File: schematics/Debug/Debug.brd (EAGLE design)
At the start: 100 x 80 mm, 12 parts

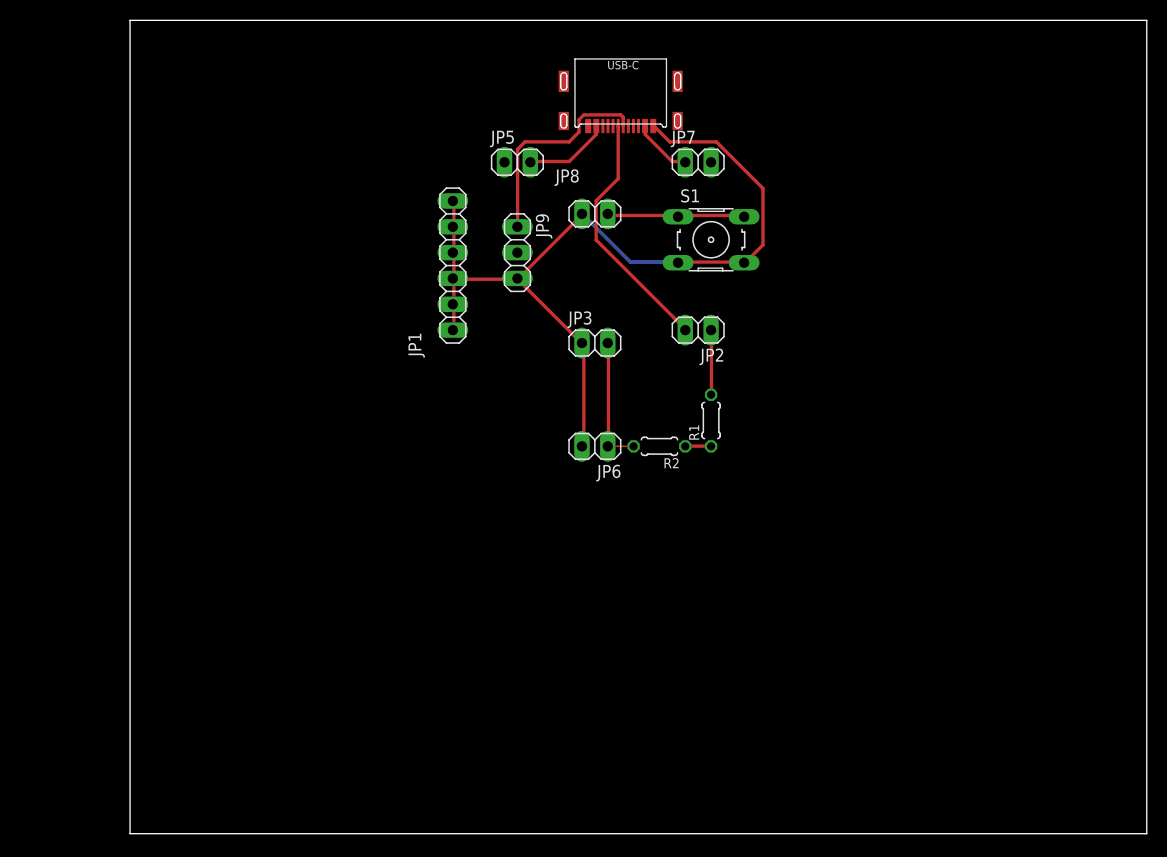
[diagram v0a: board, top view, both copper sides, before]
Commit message: Debug plata
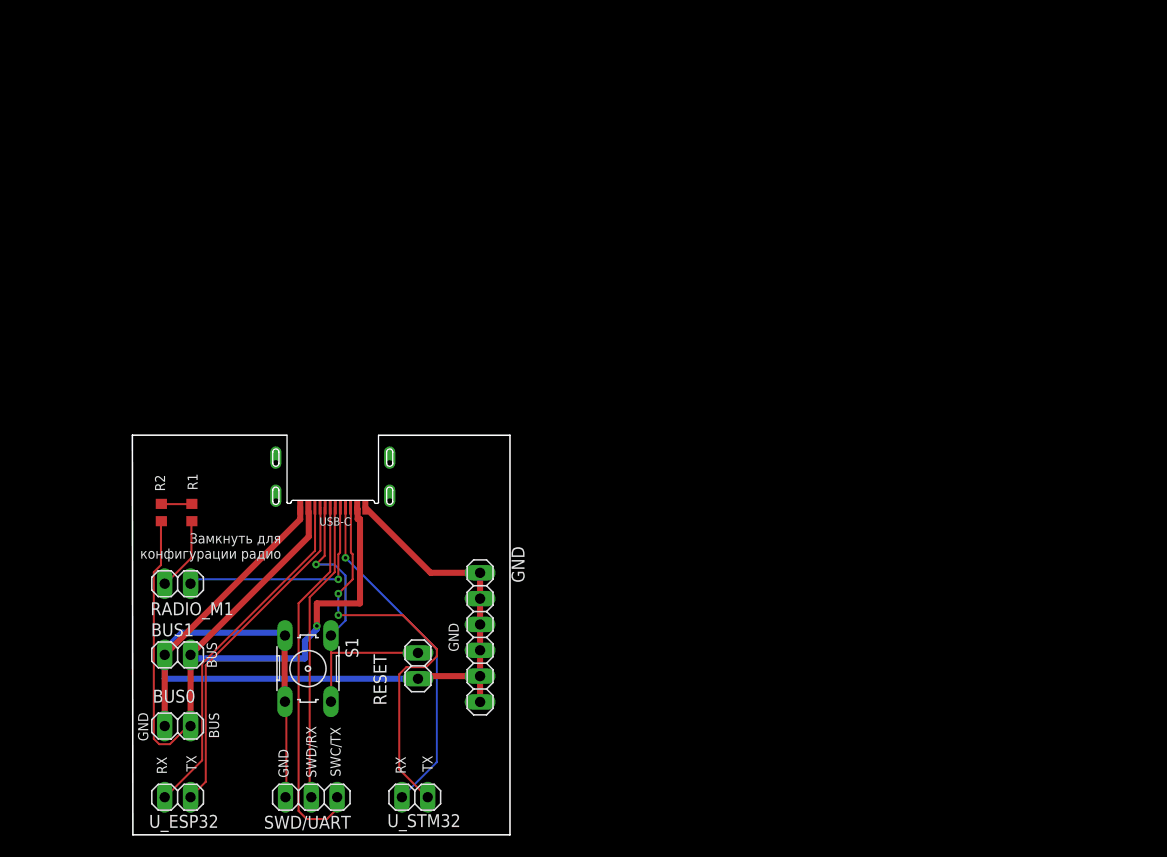
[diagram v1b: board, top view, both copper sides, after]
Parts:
- removed JP1: (no value), pinhead:1X06
- removed JP2, JP3, JP5, JP6, JP7, JP8: (no value), pinhead:1X02
- removed JP9: (no value), pinhead:1X03
- added BUS0, BUS1, RADIO_M1, RESET, U_ESP32, U_STM32: (no value), pinhead:1X02
- added GND: (no value), pinhead:1X06
- added SWD/UART: (no value), pinhead:1X03
- R1, R2: device resistor:0204/5 -> rcl:R0603
- moved S1 57.9 mm to (17.5, 16.2), turned to 270 degrees
- moved R1 51.9 mm to (6.08, 31.6), turned to 270 degrees
- moved R2 49.4 mm to (3.08, 31.6), turned to 270 degrees
- moved U$1 46.6 mm to (19.9, 39.2)
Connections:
- removed net N$1: JP5.2, U$1.TX1
- removed net N$10: JP1.1, JP1.2, JP1.3, JP1.4, JP1.5, JP1.6, JP3.1, JP6.2, JP8.1, JP9.3, S1.3, S1.4, U$1.GND0, U$1.GND1
- removed net N$11: JP9.2, U$1.SWDIO
- removed net N$12: JP9.1, U$1.SWDCLK
- removed net N$2: JP5.1, U$1.RX1
- removed net N$3: JP7.1, U$1.RX0
- removed net N$4: JP8.2, S1.1, S1.2, U$1.P$6
- removed net N$5: JP7.2, U$1.TX0
- removed net N$6: JP3.2, JP6.1, R2.2, U$1.VBUS0, U$1.VBUS1
- removed net N$9: JP2.2, U$1.M1
- new net BUS: BUS0.1, BUS1.2, R2.2, U$1.BUS0, U$1.BUS1
- new net GND: BUS0.2, BUS1.1, GND.1, GND.2, GND.3, GND.4, GND.5, GND.6, RESET.1, S1.3, S1.4, SWD/UART.3, U$1.GND0, U$1.GND1
- new net M1: RADIO_M1.2, U$1.M1
- new net RESET: RESET.2, S1.1, S1.2, U$1.RESET
- new net RX+: U$1.RX1, U_ESP32.1
- new net RX-: U$1.RX0, U_STM32.1
- new net SWC: SWD/UART.1, U$1.SWC
- new net SWD: SWD/UART.2, U$1.SWD
- new net TX+: U$1.TX1, U_ESP32.2
- new net TX-: U$1.TX0, U_STM32.2
- net N$7: now also RADIO_M1.1; no longer JP2.1
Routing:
- net GND: track 0.00 -> 117.0 mm
- net N$10: track 87.3 -> 0.00 mm
- net BUS: track 0.00 -> 83.8 mm, vias 0 -> 1
- net TX-: track 0.00 -> 40.7 mm, vias 0 -> 2
- net SWC: track 0.00 -> 36.8 mm
- net RX+: track 0.00 -> 34.6 mm
- net TX+: track 0.00 -> 33.8 mm
- net RX-: track 0.00 -> 33.6 mm, vias 0 -> 1
- net RESET: track 0.00 -> 30.9 mm, vias 0 -> 1
- net SWD: track 0.00 -> 29.6 mm
- net N$9: track 24.6 -> 0.00 mm
- net M1: track 0.00 -> 21.9 mm, vias 0 -> 1
- net N$12: track 21.1 -> 0.00 mm
- net N$4: track 13.7 -> 0.00 mm
- net N$6: track 12.8 -> 0.00 mm
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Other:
- board size 100 x 80 mm -> 37.1 x 39.3 mm
- board text added: "BUS"
- board text added: "GND"
- board text added: "RX"
- board text added: "SWC/TX"
- board text added: "SWD/RX"
- board text added: "TX"
- board text added: "Замкнуть для конфигурации радио"

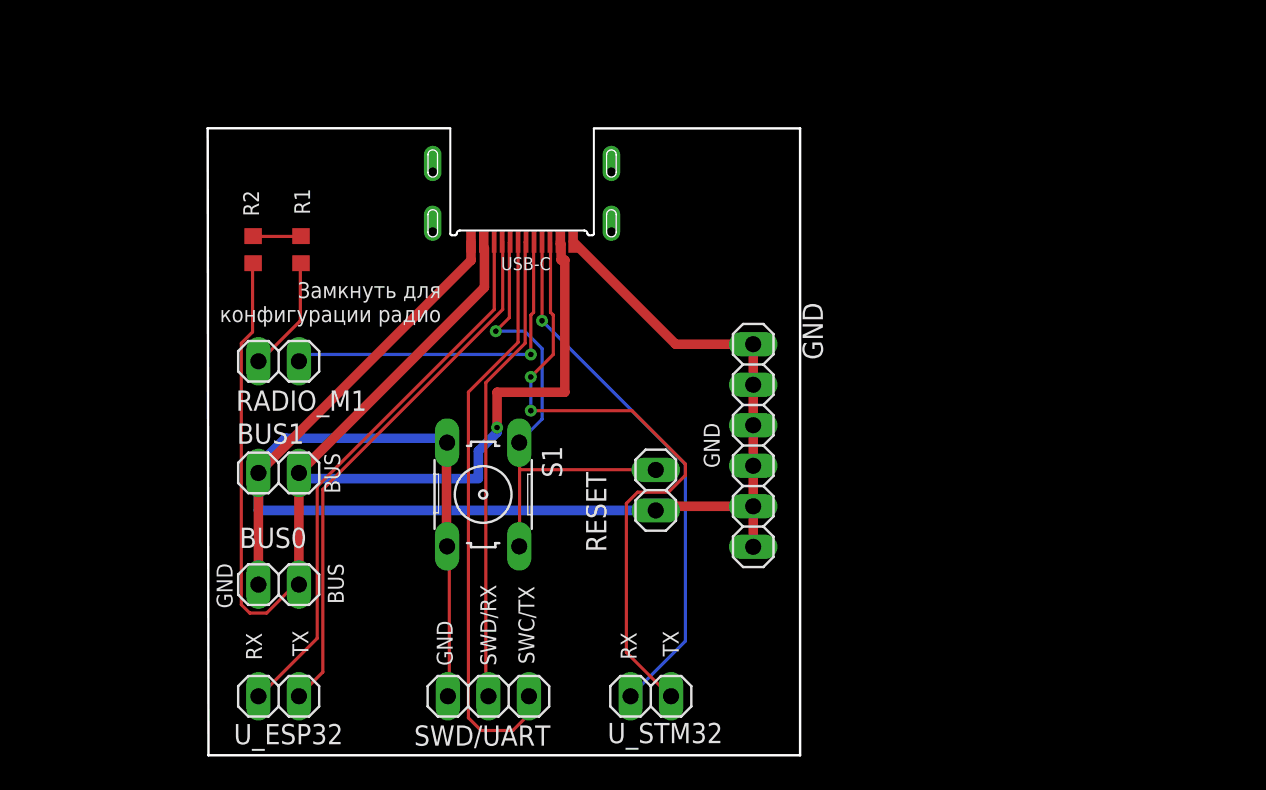
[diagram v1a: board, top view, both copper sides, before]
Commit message: Очередная дебажная плата
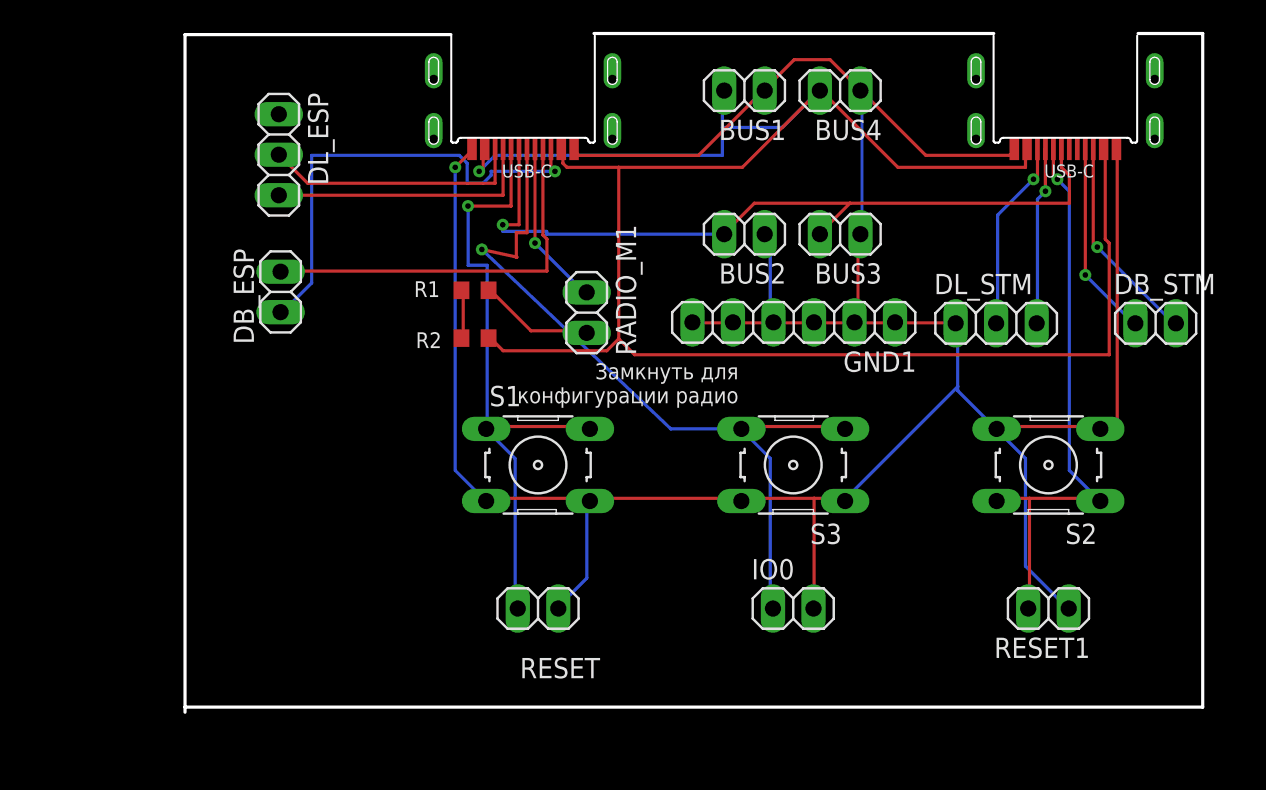
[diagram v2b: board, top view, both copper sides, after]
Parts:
- removed BUS0, U_ESP32, U_STM32: (no value), pinhead:1X02
- removed GND: (no value), pinhead:1X06
- removed SWD/UART: (no value), pinhead:1X03
- added BUS2, BUS3, BUS4, DB_ESP, DB_STM, IO0, RESET1: (no value), pinhead:1X02
- added DL_ESP, DL_STM: (no value), pinhead:1X03
- added GND1: (no value), pinhead:1X06
- added S2, S3: (no value), switch-omron:B3F-10XX
- added U$2: USB-C, CanCubeSat:USB-C
- moved BUS1 37.8 mm to (33.9, 41.6), turned to 180 degrees
- moved RADIO_M1 19.5 mm to (24.0, 27.6), turned to 90 degrees
- moved R2 15.0 mm to (17.0, 26.0), turned to 0 degrees
- moved R1 11.2 mm to (17.0, 29.0), turned to 0 degrees
- moved RESET 10.5 mm to (20.9, 9.09), turned to 180 degrees
- moved U$1 5.81 mm to (20.0, 45.0)
- moved S1 3.91 mm to (20.9, 18.1), turned to 0 degrees
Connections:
- removed net RX+: U$1.RX1, U_ESP32.1
- removed net RX-: U$1.RX0, U_STM32.1
- removed net SWC: SWD/UART.1, U$1.SWC
- removed net SWD: SWD/UART.2, U$1.SWD
- removed net TX+: U$1.TX1, U_ESP32.2
- removed net TX-: U$1.TX0, U_STM32.2
- new net 3V3: BUS2.2, BUS3.2, U$1.SWC, U$2.SWC
- new net N$3: IO0.1, S3.3, S3.4, U$1.SWD
- new net RESET_STM: RESET1.2, S2.1, S2.2, U$2.RESET
- new net RX0: DB_ESP.1, U$1.RX0
- new net RX0_STM: DB_STM.1, U$2.RX0
- new net RX1: DL_ESP.2, U$1.RX1
- new net SWC_STM: DL_STM.3, U$2.TX1
- new net SWD_STM: DL_STM.2, U$2.RX1
- new net TX0: DB_ESP.2, U$1.TX0
- new net TX0_STM: DB_STM.2, U$2.TX0
- new net TX1: DL_ESP.3, U$1.TX1
- net BUS: now also BUS4.2, U$2.BUS0, U$2.BUS1; no longer BUS0.1
- net GND: now also BUS2.1, BUS3.1, BUS4.1, DL_STM.1, GND1.1, GND1.2, GND1.3, GND1.4, GND1.5, GND1.6, IO0.2, RESET1.1, S2.3, S2.4, S3.1, S3.2, U$2.GND0, U$2.GND1; no longer BUS0.2, GND.1, GND.2, GND.3, GND.4, GND.5, GND.6, SWD/UART.3
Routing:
- net GND: track 117.0 -> 187.2 mm, vias 0 -> 1
- net N$3: track 0.00 -> 49.2 mm, vias 0 -> 1
- net 3V3: track 0.00 -> 49.0 mm, vias 0 -> 1
- net BUS: track 83.8 -> 127.4 mm
- net TX-: track 40.7 -> 0.00 mm, vias 2 -> 0
- net RESET_STM: track 0.00 -> 37.1 mm, vias 0 -> 1
- net SWC: track 36.8 -> 0.00 mm
- net RX+: track 34.6 -> 0.00 mm
- net TX+: track 33.8 -> 0.00 mm
- net RX-: track 33.6 -> 0.00 mm, vias 1 -> 0
- net SWD: track 29.6 -> 0.00 mm
- net TX0: track 0.00 -> 29.5 mm, vias 0 -> 1
- net RX0: track 0.00 -> 24.5 mm
- net TX1: track 0.00 -> 17.0 mm
- net RX1: track 0.00 -> 16.4 mm
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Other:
- board size 37.1 x 39.3 mm -> 63.8 x 42.5 mm
- board text removed: "BUS"
- board text removed: "GND"
- board text removed: "RX"
- board text removed: "SWC/TX"
- board text removed: "SWD/RX"
- board text removed: "TX"

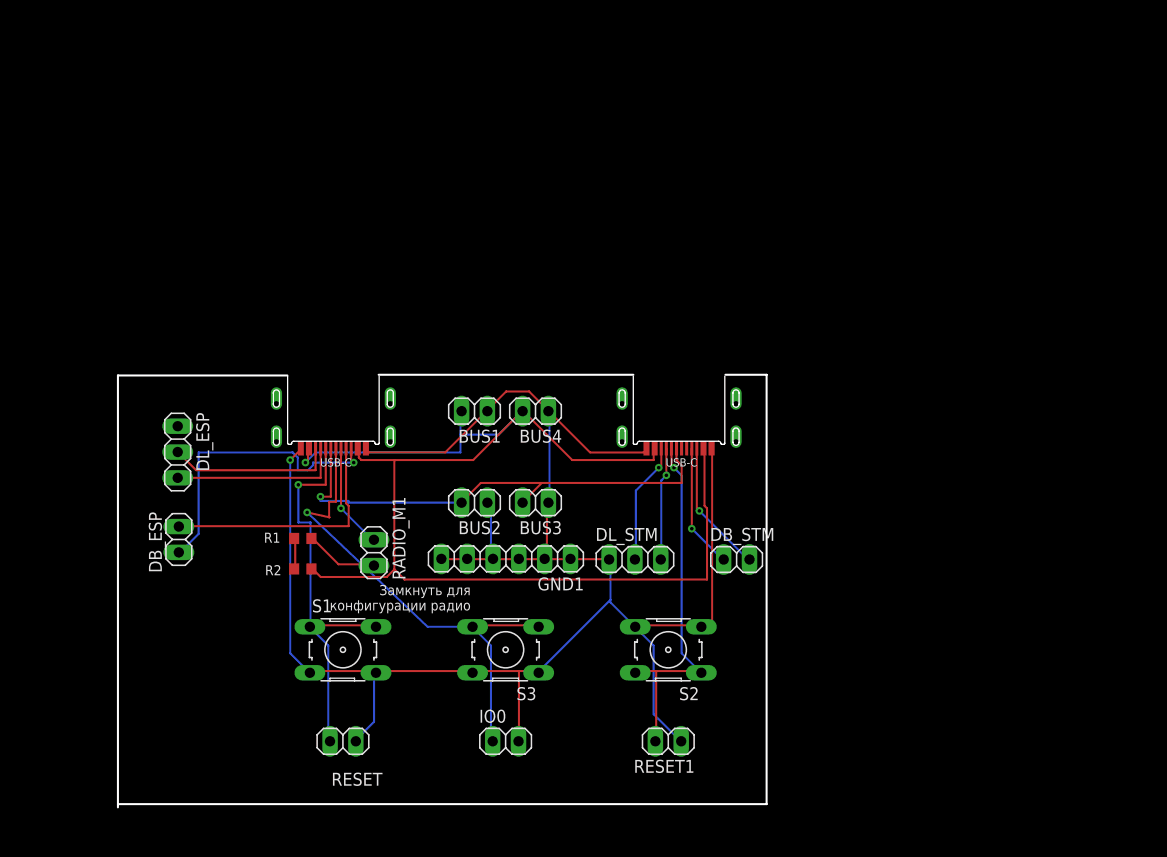
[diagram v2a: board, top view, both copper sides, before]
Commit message: Отладочная плата v2
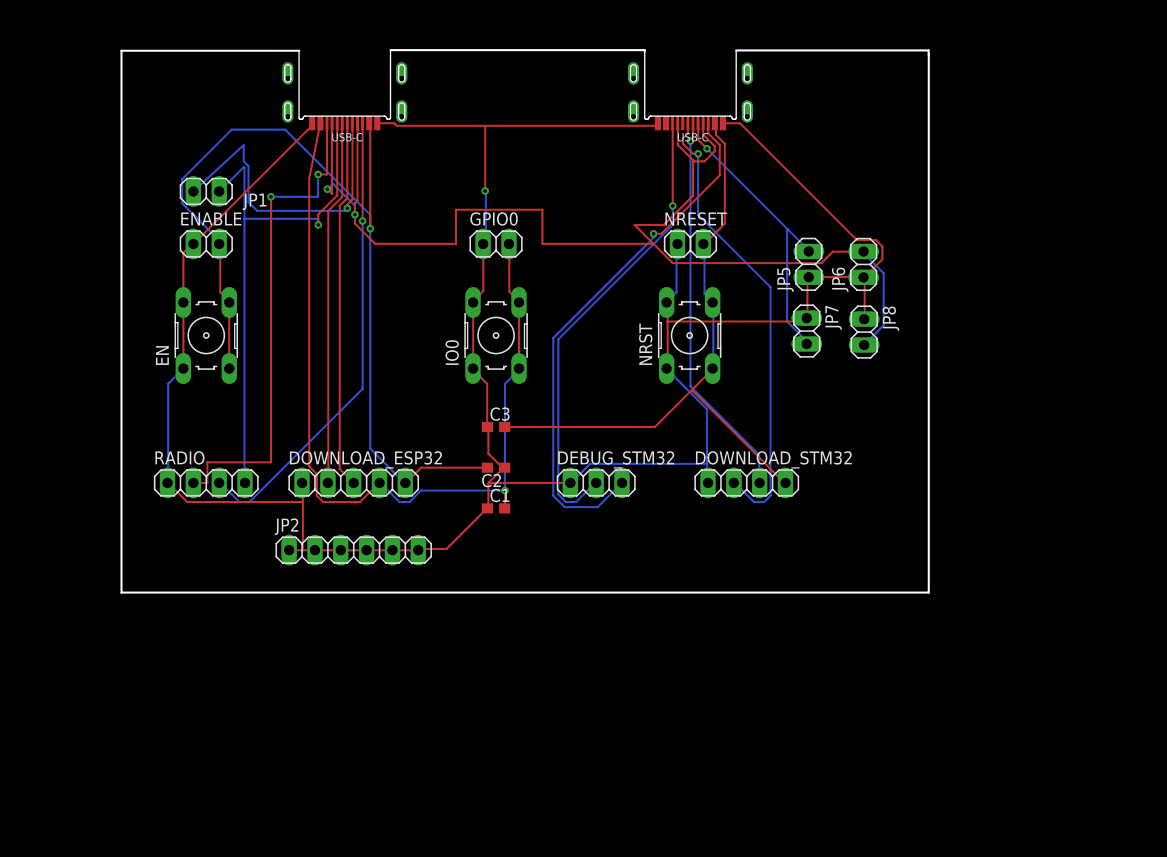
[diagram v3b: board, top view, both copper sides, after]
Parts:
- removed BUS1, BUS2, BUS3, BUS4, DB_ESP, DB_STM, RADIO_M1, RESET, RESET1: (no value), pinhead:1X02
- removed DL_ESP, DL_STM: (no value), pinhead:1X03
- removed GND1: (no value), pinhead:1X06
- removed R1: 1k, rcl:R0603
- removed R2: 10k, rcl:R0603
- removed S1, S2, S3: (no value), switch-omron:B3F-10XX
- added C1, C2, C3: 1nF, rcl:C0603
- added DEBUG_STM32: (no value), pinhead:1X03
- added DOWNLOAD_ESP32: (no value), pinhead:1X05
- added DOWNLOAD_STM32, RADIO: (no value), pinhead:1X04
- added EN, NRST: (no value), switch-omron:B3F-10XX
- added ENABLE, GPIO0, JP1, JP5, JP6, JP7, JP8, NRESET: (no value), pinhead:1X02
- added JP2: (no value), pinhead:1X06
- IO0: device pinhead:1X02 -> switch-omron:B3F-10XX
- moved IO0 39.9 mm to (36.0, 49.0), turned to 90 degrees
- moved U$1 32.0 mm to (21.1, 77.0)
- moved U$2 32.0 mm to (55.1, 77.0)
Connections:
- removed net N$3: IO0.1, S3.3, S3.4, U$1.SWD
- removed net N$7: R1.2, RADIO_M1.1
- removed net N$8: R1.1, R2.1
- removed net RESET: RESET.2, S1.1, S1.2, U$1.RESET
- removed net RESET_STM: RESET1.2, S2.1, S2.2, U$2.RESET
- removed net RX0: DB_ESP.1, U$1.RX0
- removed net RX0_STM: DB_STM.1, U$2.RX0
- removed net SWC_STM: DL_STM.3, U$2.TX1
- removed net SWD_STM: DL_STM.2, U$2.RX1
- removed net TX0: DB_ESP.2, U$1.TX0
- removed net TX0_STM: DB_STM.2, U$2.TX0
- new net 3V3-S: JP1.1, U$1.NC/3V3
- new net EN: C2.2, DOWNLOAD_ESP32.5, EN.3, EN.4, ENABLE.2, U$1.NRST/EN
- new net IO0: C1.2, DOWNLOAD_ESP32.4, GPIO0.2, IO0.3, IO0.4, U$1.NC/GPIO
- new net NRST: C3.2, DOWNLOAD_STM32.4, NRESET.2, NRST.3, NRST.4, U$2.NRST/EN
- new net RX: DEBUG_STM32.3, U$2.RX0
- new net RXD: DOWNLOAD_ESP32.3, U$1.SWD/RXD
- new net SWC: DOWNLOAD_STM32.2, U$2.SWC/TXD
- new net SWD: DOWNLOAD_STM32.3, U$2.SWD/RXD
- new net TX: DEBUG_STM32.2, U$2.TX0
- new net TXD: DOWNLOAD_ESP32.2, U$1.SWC/TXD
- net 3V3: now also JP5.2, JP7.2, U$2.NC/3V3; no longer BUS2.2, BUS3.2, U$1.SWC, U$2.SWC
- net BUS: now also JP6.2, JP8.2, U$1.3V3/BUS0, U$1.3V3/BUS1, U$2.3V3/BUS0, U$2.3V3/BUS1; no longer BUS1.2, BUS4.2, R2.2, U$1.BUS0, U$1.BUS1, U$2.BUS0, U$2.BUS1
- net GND: now also C1.1, C2.1, C3.1, DEBUG_STM32.1, DOWNLOAD_ESP32.1, DOWNLOAD_STM32.1, EN.1, EN.2, ENABLE.1, GPIO0.1, IO0.1, JP2.1, JP2.2, JP2.3, JP2.4, JP2.5, JP2.6, JP5.1, JP6.1, JP7.1, JP8.1, NRESET.1, NRST.1, NRST.2, RADIO.1; no longer BUS1.1, BUS2.1, BUS3.1, BUS4.1, DL_STM.1, GND1.1, GND1.2, GND1.3, GND1.4, GND1.5, GND1.6, RESET.1, RESET1.1, S1.3, S1.4, S2.3, S2.4, S3.1, S3.2
- net M1: now also JP1.2, RADIO.4, U$1.NC/M1; no longer RADIO_M1.2, U$1.M1
- net RX1: now also RADIO.3, U$1.RX0; no longer DL_ESP.2, U$1.RX1
- net TX1: now also RADIO.2, U$1.TX0; no longer DL_ESP.3, U$1.TX1
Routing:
- net EN: track 0.00 -> 91.6 mm, vias 0 -> 1
- net IO0: track 0.00 -> 84.9 mm, vias 0 -> 1
- net GND: track 187.2 -> 252.2 mm
- net NRST: track 0.00 -> 62.0 mm
- net RX: track 0.00 -> 52.5 mm, vias 0 -> 1
- net N$3: track 49.2 -> 0.00 mm, vias 1 -> 0
- net TX: track 0.00 -> 46.0 mm, vias 0 -> 1
- net SWC: track 0.00 -> 45.4 mm, vias 0 -> 1
- net M1: track 10.4 -> 53.2 mm
- net RESET: track 40.2 -> 0.00 mm, vias 1 -> 0
- net SWD: track 0.00 -> 38.3 mm, vias 0 -> 1
- net RESET_STM: track 37.1 -> 0.00 mm, vias 1 -> 0
- net RXD: track 0.00 -> 36.3 mm
- net TXD: track 0.00 -> 36.0 mm
- net TX1: track 17.0 -> 48.5 mm, vias 0 -> 2
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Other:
- board size 63.8 x 42.5 mm -> 79.4 x 53.3 mm
- board text removed: "Замкнуть для конфигурации радио"
